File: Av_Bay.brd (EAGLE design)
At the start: 120.3 x 36.8 mm, 9 parts

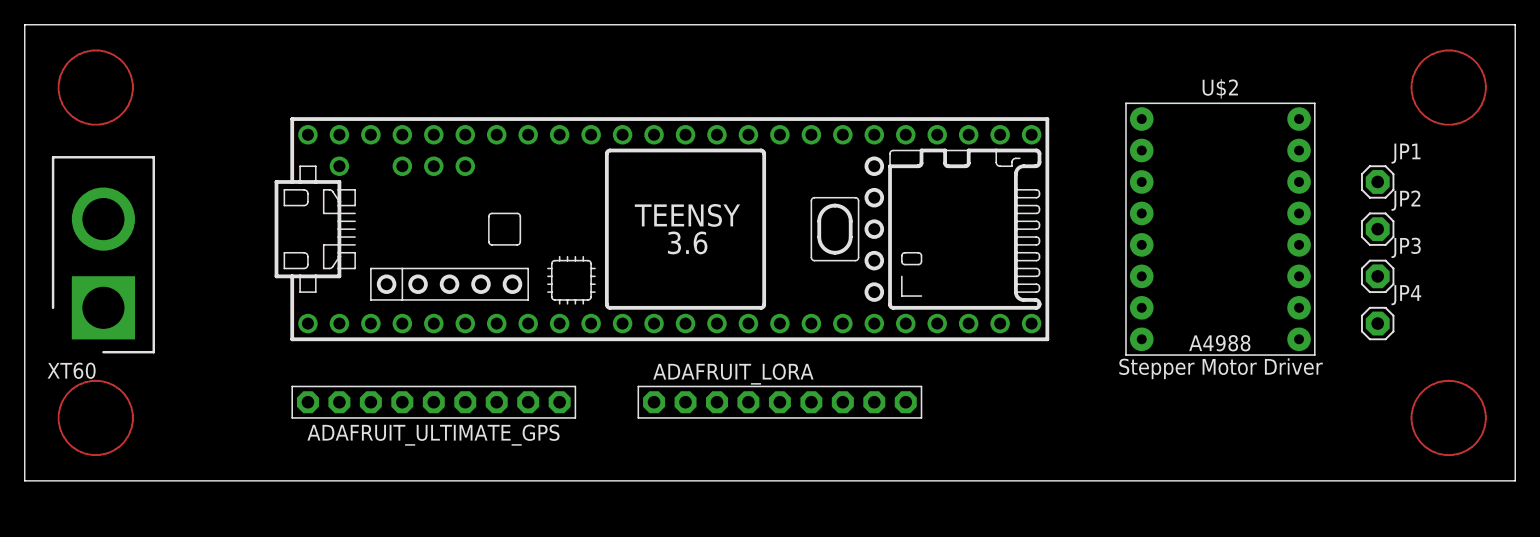
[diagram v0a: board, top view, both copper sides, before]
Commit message: Add files via upload
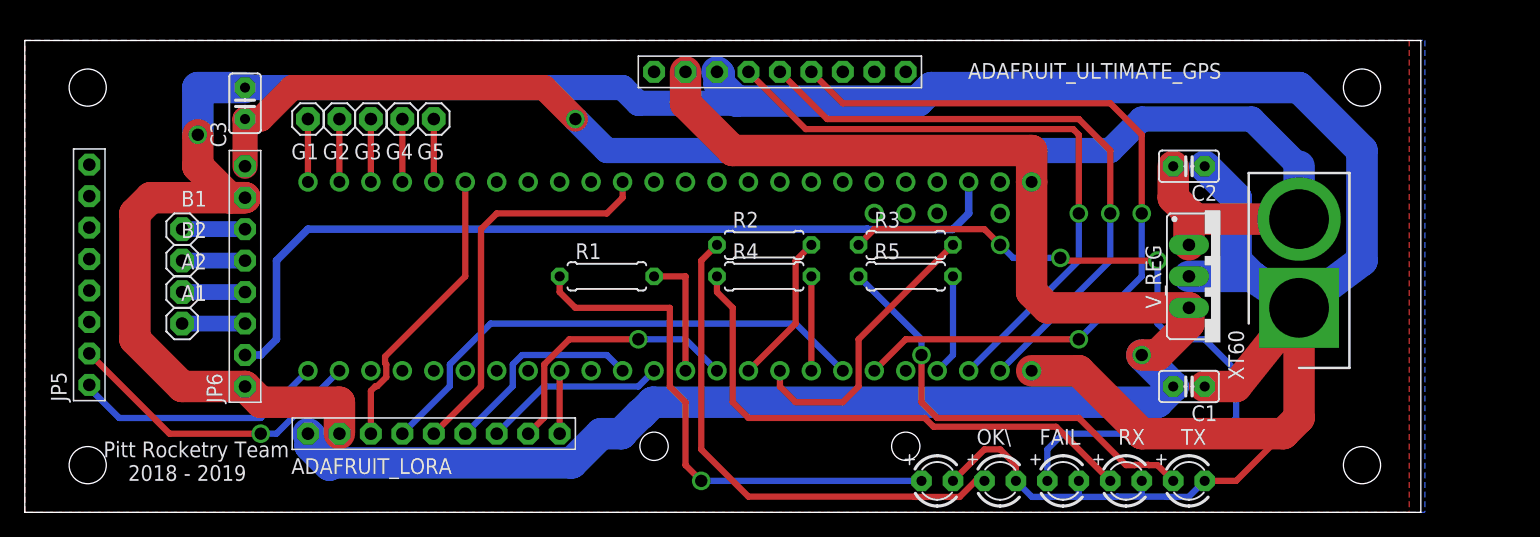
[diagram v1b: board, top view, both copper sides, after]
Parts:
- removed JP1, JP2, JP3, JP4: (no value), adafruit:1X01
- removed U$2: A4988_STEP, IC:A4988_STEP
- added A1, A2, B1, B2, G1, G2, G3, G4, G5: (no value), adafruit:1X01
- added C1, C2, C3: (no value), adafruit:C025-025X050
- added FAIL, LED5, OK\, RX, TX: (no value), adafruit:LED3MM
- added JP5, JP6: (no value), adafruit:1X08-BIG
- added R1, R2, R3, R4, R5: (no value), adafruit:0207/7
- added V_REG: (no value), v-reg:317TS
- moved XT60 96.5 mm to (104.1, 55.9)
- moved ADAFRUIT_ULTIMATE_GPS 38.6 mm to (62.2, 76.2)
- moved ADAFRUIT_LORA 28.1 mm to (34.3, 47.0)
- moved U$1 4.58 mm to (54.6, 59.7), flipped to the bottom
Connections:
- removed net 1A: JP3.1, U$2.1A
- removed net 1B: JP4.1, U$2.1B
- removed net 2A: JP2.1, U$2.2A
- removed net 2B: JP1.1, U$2.2B
- removed net 5V: ADAFRUIT_ULTIMATE_GPS.8
- removed net EN: ADAFRUIT_ULTIMATE_GPS.2, U$1.2
- removed net MASTER_BATT: XT60.2
- removed net N$10: U$2./RST, U$2./SLP
- removed net PPS: ADAFRUIT_ULTIMATE_GPS.9, U$1.3/CANTX
- new net 5V_SUPP: ADAFRUIT_LORA.1, ADAFRUIT_ULTIMATE_GPS.8, C1.2, U$1.VIN, V_REG.3
- new net A1: A1.1, JP6.3
- new net A2: A2.1, JP6.4
- new net B1: B1.1, JP6.6
- new net B2: B2.1, JP6.5
- new net ERR_LED: R3.2, U$1.7
- new net EXTRA_LED: R1.2, U$1.10/CS
- new net FAULT: JP6.2, U$1.3V3_LO
- new net G1: G1.1, U$1.33/A14
- new net G2: G2.1, U$1.34/A15
- new net G3: G3.1, U$1.35/A16
- new net G4: G4.1, U$1.36/A17
- new net G5: G5.1, U$1.37/A18
- new net GPS_3.3V: ADAFRUIT_ULTIMATE_GPS.1
- new net MASTER_BATT_IN: C2.2, C3.1, JP6.8, V_REG.1, XT60.2
- new net N$1: R5.1, TX.A
- new net N$4: OK\.A, R2.1
- new net N$5: JP5.3
- new net N$6: LED5.A, R1.1
- new net OK_LED: R2.2, U$1.8
- new net RX_LED: R4.2, U$1.6
- new net TX_LED: R5.2, U$1.2
- net CS: now also U$1.9/CS; no longer U$1.24
- net DIR: now also JP5.1; no longer U$2.DIR
- net EN_LORA: now also U$1.38/A19
- net GND: now also C1.1, C2.1, C3.2, FAIL.K, JP6.1, JP6.7, LED5.K, OK\.K, RX.K, TX.K, V_REG.2; no longer U$2.GND, U$2.GND2
- net LOGIC_POWER: no longer U$2.VDD
- net N$2: now also R4.1, RX.A; no longer U$1.7
- net N$3: now also FAIL.A, R3.1; no longer U$1.8
- net RST: now also U$1.24; no longer U$1.25
- net RX: now also U$1.1/TX; no longer U$1.0/RX
- net SCK: now also U$1.13/SCK; no longer U$1.6
- net STEP: now also JP5.2; no longer U$2.STEP
- net TX: now also U$1.0/RX; no longer U$1.1/TX
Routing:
- net GND: track 0.00 -> 266.0 mm, vias 0 -> 1
- net 5V_SUPP: track 0.00 -> 140.5 mm, vias 0 -> 1
- net MASTER_BATT_IN: track 0.00 -> 114.9 mm, vias 0 -> 1
- net FAULT: track 0.00 -> 69.4 mm
- net FIX: track 0.00 -> 65.0 mm, vias 0 -> 2
- net N$3: track 0.00 -> 61.4 mm, vias 0 -> 3
- net RX: track 0.00 -> 51.5 mm, vias 0 -> 1
- net TX: track 0.00 -> 50.8 mm, vias 0 -> 1
- net N$2: track 0.00 -> 43.8 mm
- net N$6: track 0.00 -> 43.5 mm, vias 0 -> 1
- net N$4: track 0.00 -> 42.0 mm
- net G0: track 0.00 -> 41.9 mm
- net N$1: track 0.00 -> 35.2 mm, vias 0 -> 1
- net SCK: track 0.00 -> 31.8 mm
- net STEP: track 0.00 -> 25.0 mm, vias 0 -> 1
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- added copper zone on layer 1, net GND
- added copper zone on layer 16, net GND
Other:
- board size 120.3 x 36.8 mm -> 112.7 x 38.1 mm
- board text added: "Pitt Rocketry Team 2018 - 2019"
